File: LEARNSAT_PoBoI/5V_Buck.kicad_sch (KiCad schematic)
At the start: 22 parts, among them U8 LT1616ES6#TRMPBF, U9 LT1616ES6#TRMPBF

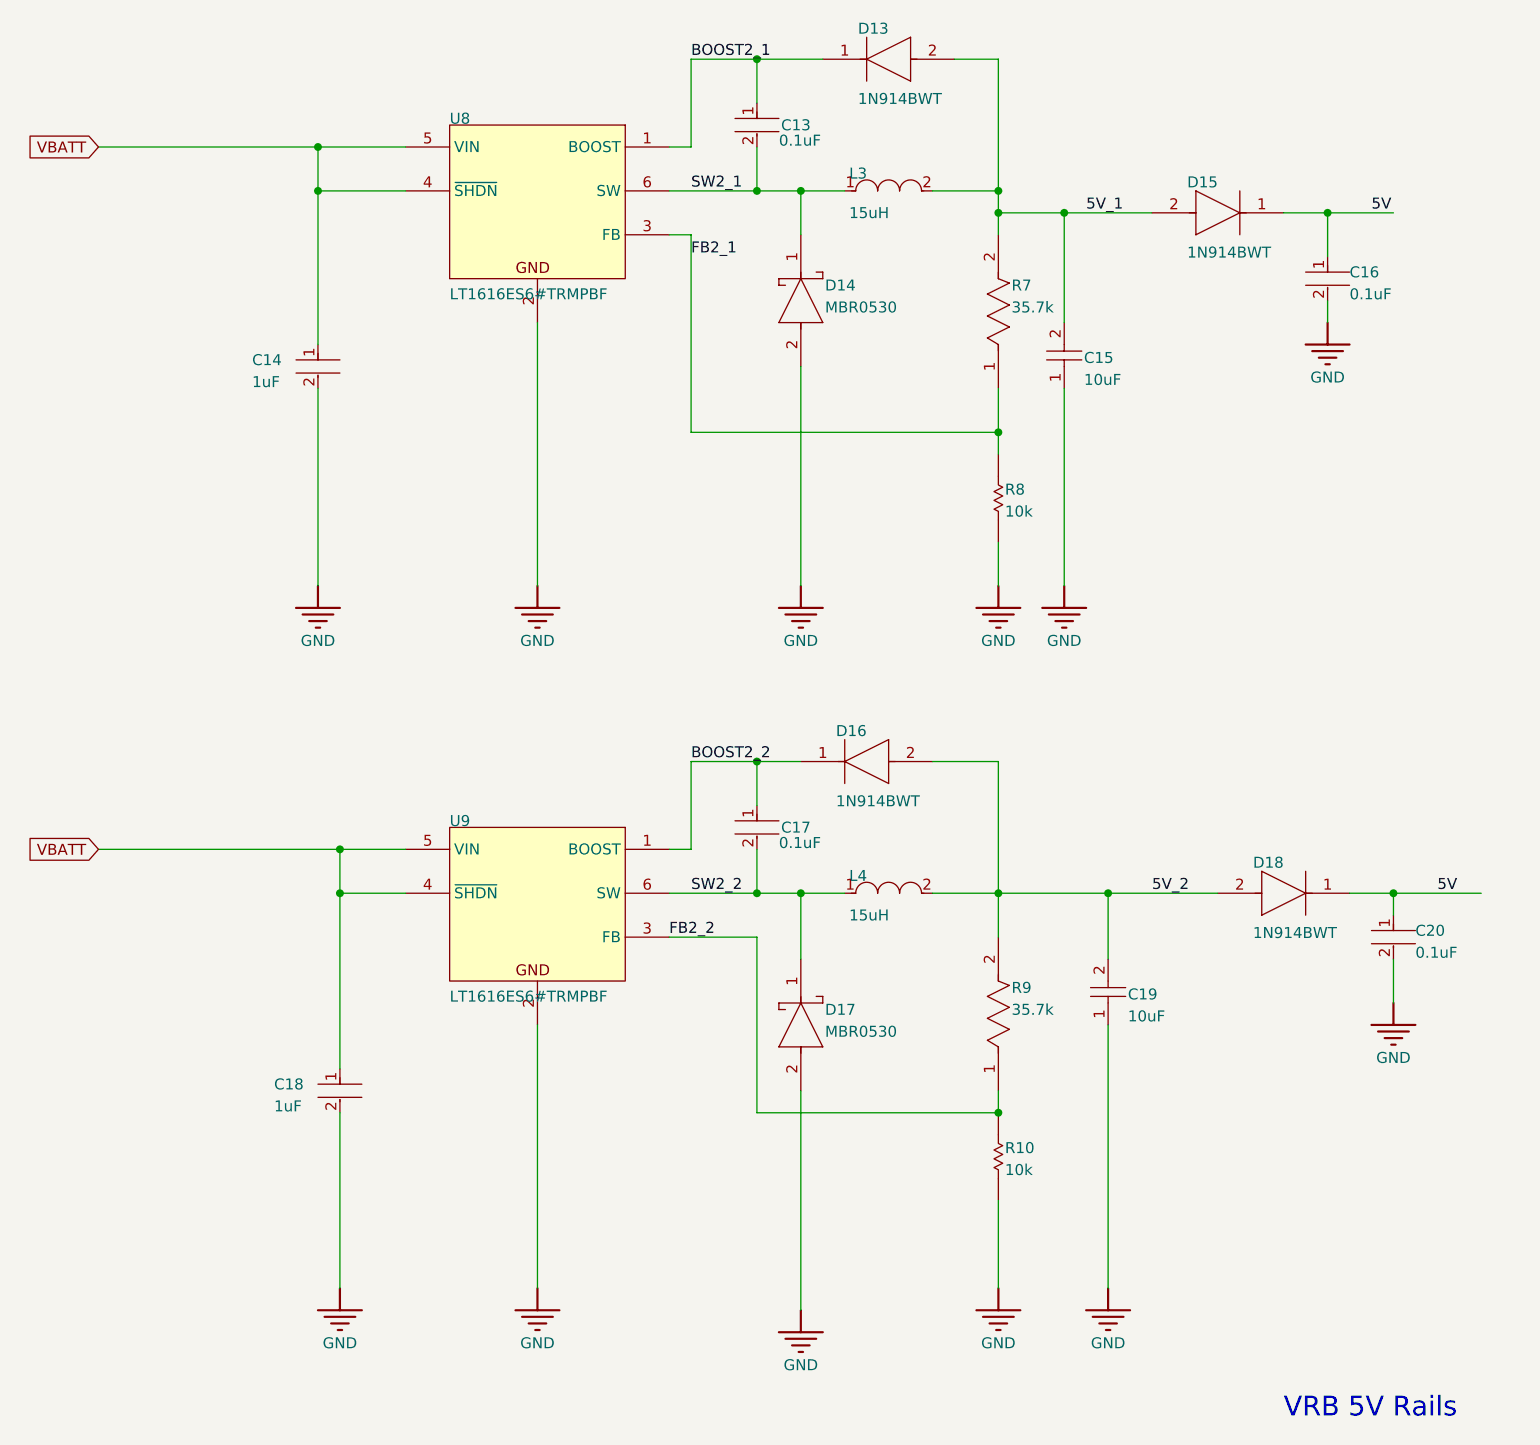
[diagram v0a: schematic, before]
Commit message: Added footprints
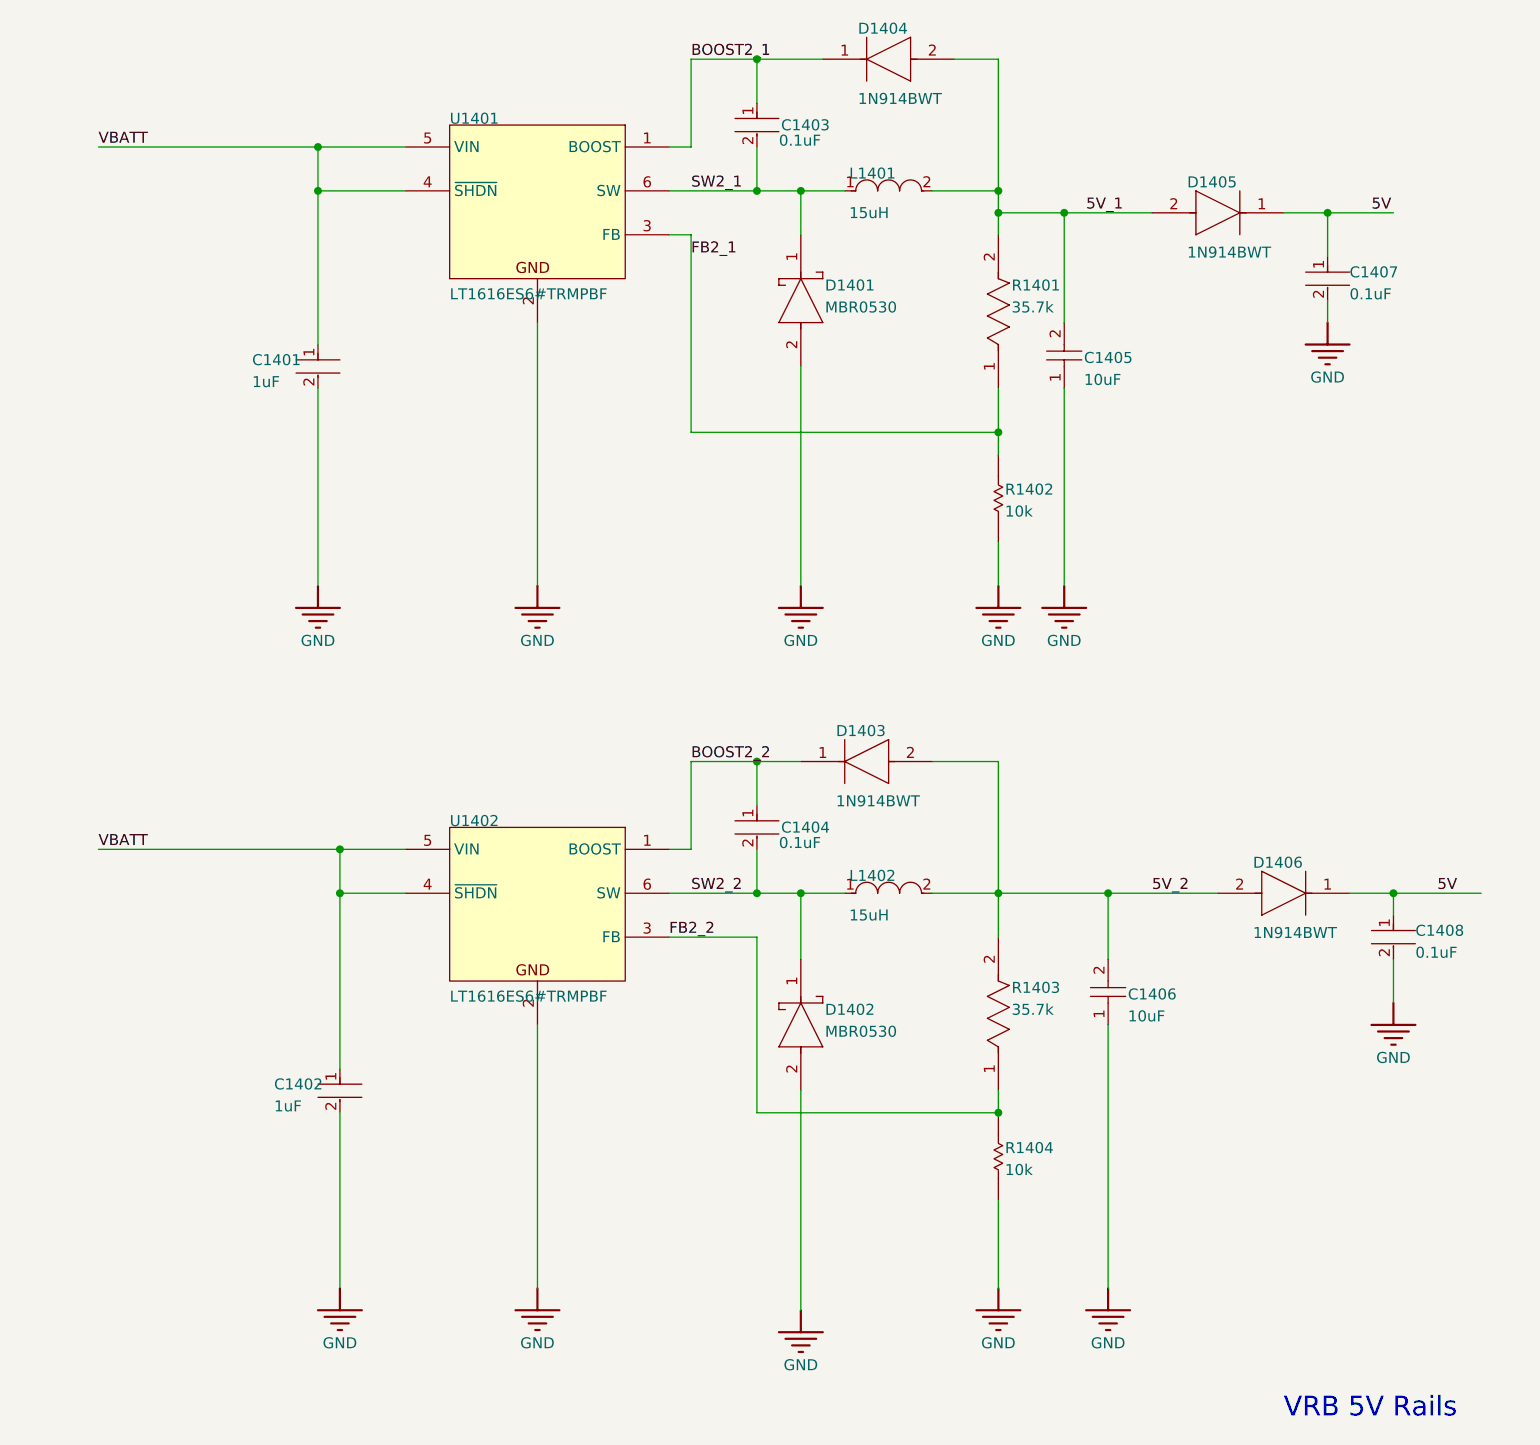
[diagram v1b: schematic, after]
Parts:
- C1401: renamed from C14; footprint FP-CL10-IPC_B -> Capacitor_SMD:C_0603_1608Metric
- C1402: renamed from C18; footprint FP-CL10-IPC_B -> Capacitor_SMD:C_0603_1608Metric
- C1403: renamed from C13; footprint FP-C0603-CJ-MFG -> Capacitor_SMD:C_0603_1608Metric
- C1404: renamed from C17; footprint FP-C0603-CJ-MFG -> Capacitor_SMD:C_0603_1608Metric
- C1405: renamed from C15; footprint CAPC0603(1608)100_L -> Capacitor_SMD:C_0603_1608Metric
- C1406: renamed from C19; footprint CAPC0603(1608)100_L -> Capacitor_SMD:C_0603_1608Metric
- C1407: renamed from C16; footprint FP-C0603-CJ-MFG -> Capacitor_SMD:C_0603_1608Metric
- C1408: renamed from C20; footprint FP-C0603-CJ-MFG -> Capacitor_SMD:C_0603_1608Metric
- D1401: renamed from D14; footprint FP-425-04-MFG -> Diode_SMD:D_SOD-123
- D1402: renamed from D17; footprint FP-425-04-MFG -> Diode_SMD:D_SOD-123
- D1403: renamed from D16; footprint FP-502-01-MFG -> Diode_SMD:D_SOD-123
- D1404: renamed from D13; footprint FP-502-01-MFG -> Diode_SMD:D_SOD-123
- D1405: renamed from D15; footprint FP-502-01-MFG -> Diode_SMD:D_SOD-123
- D1406: renamed from D18; footprint FP-502-01-MFG -> Diode_SMD:D_SOD-123
- L1401: renamed from L3; footprint FP-LQH43CN_03-MFG -> Inductor_SMD:L_1812_4532Metric
- L1402: renamed from L4; footprint FP-LQH43CN_03-MFG -> Inductor_SMD:L_1812_4532Metric
- R1401: renamed from R7; footprint FP-CRCW0603-e3-IPC_C -> Resistor_SMD:R_0603_1608Metric
- R1402: renamed from R8; footprint RESC1609X50X30NL8T20 -> Resistor_SMD:R_0603_1608Metric
- R1403: renamed from R9; footprint FP-CRCW0603-e3-IPC_C -> Resistor_SMD:R_0603_1608Metric
- R1404: renamed from R10; footprint RESC1609X50X30NL8T20 -> Resistor_SMD:R_0603_1608Metric
- U1401: renamed from U8; footprint LT-S6-6-SOT-23_M -> LT1616ES6TRMPBF:SOT-6_S
- U1402: renamed from U9; footprint LT-S6-6-SOT-23_M -> LT1616ES6TRMPBF:SOT-6_S

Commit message: Add files via upload
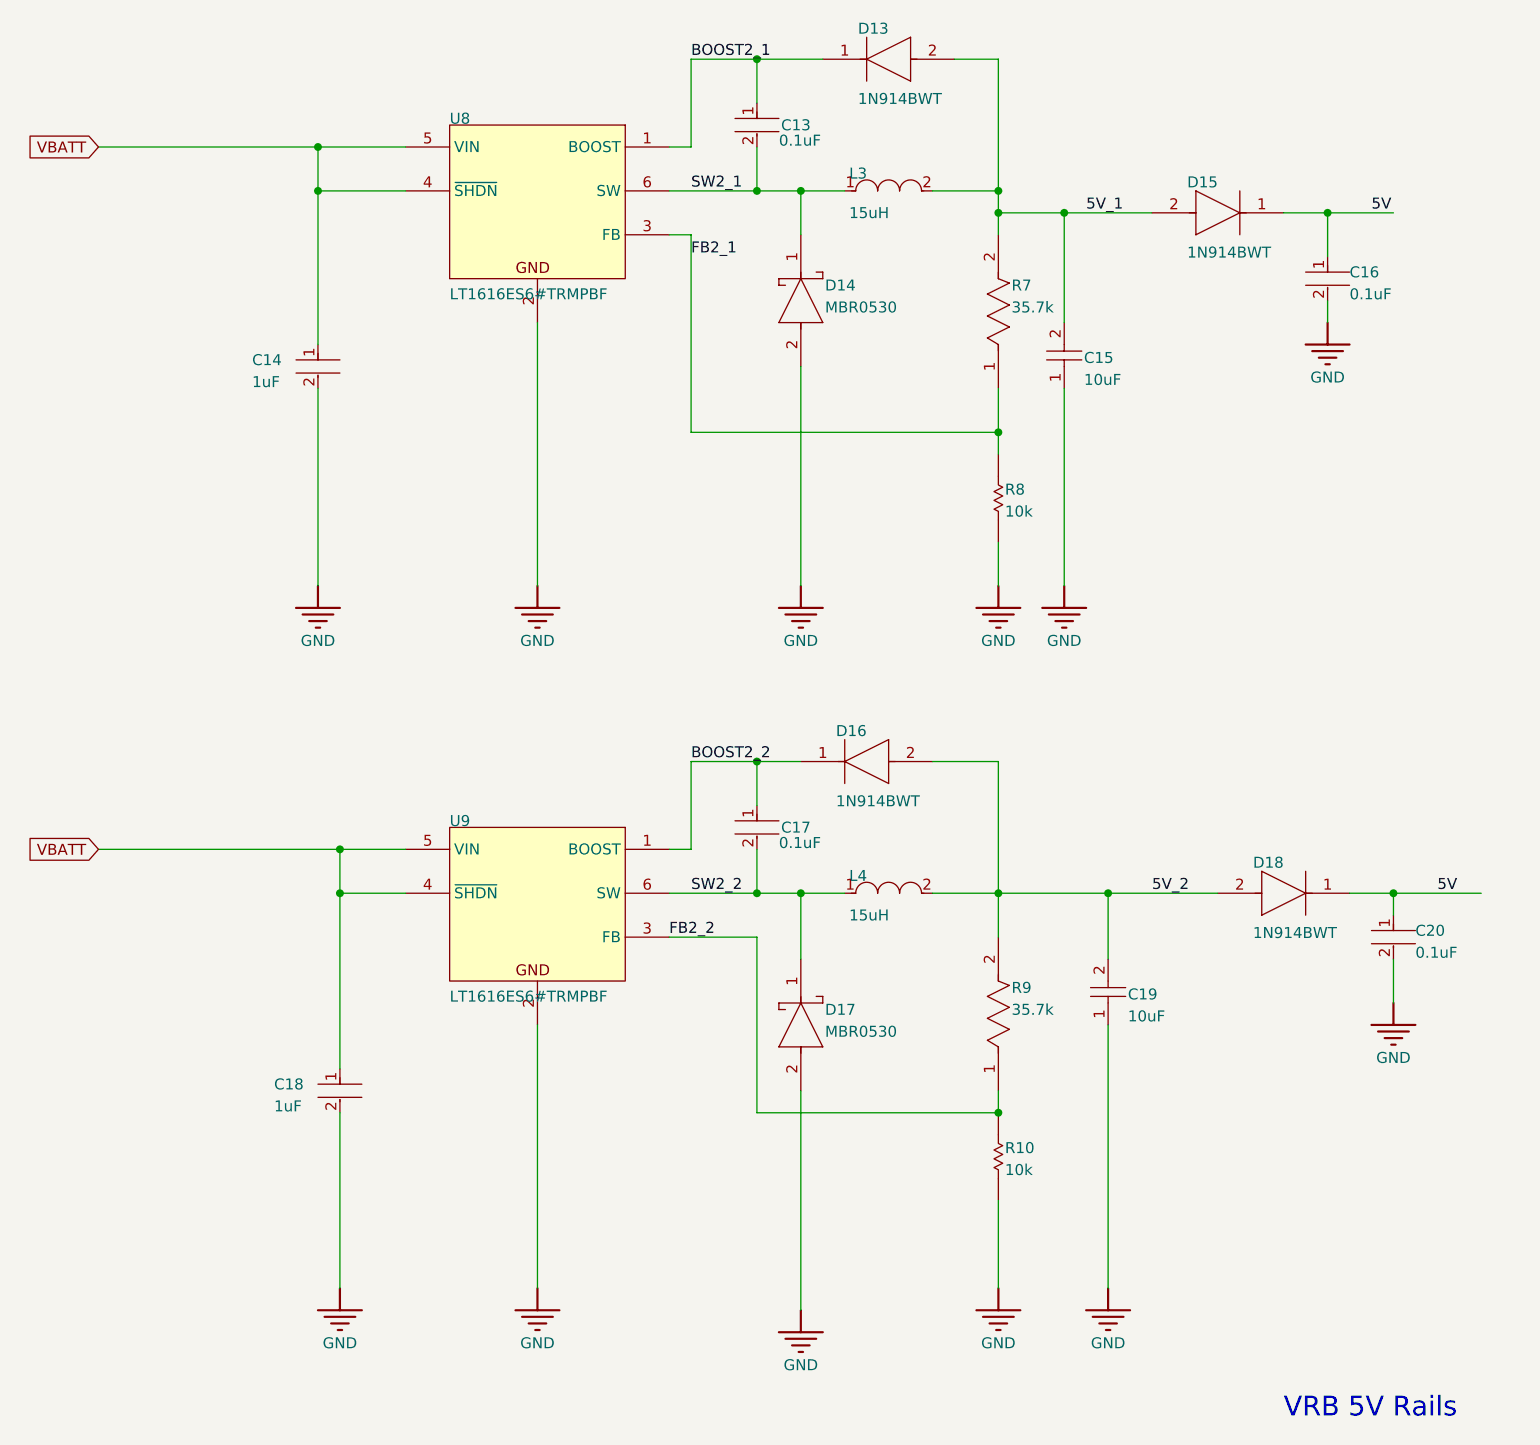
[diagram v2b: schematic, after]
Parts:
- C13: renamed from C1403; footprint Capacitor_SMD:C_0603_1608Metric -> FP-C0603-CJ-MFG
- C14: renamed from C1401; footprint Capacitor_SMD:C_0603_1608Metric -> FP-CL10-IPC_B
- C15: renamed from C1405; footprint Capacitor_SMD:C_0603_1608Metric -> CAPC0603(1608)100_L
- C16: renamed from C1407; footprint Capacitor_SMD:C_0603_1608Metric -> FP-C0603-CJ-MFG
- C17: renamed from C1404; footprint Capacitor_SMD:C_0603_1608Metric -> FP-C0603-CJ-MFG
- C18: renamed from C1402; footprint Capacitor_SMD:C_0603_1608Metric -> FP-CL10-IPC_B
- C19: renamed from C1406; footprint Capacitor_SMD:C_0603_1608Metric -> CAPC0603(1608)100_L
- C20: renamed from C1408; footprint Capacitor_SMD:C_0603_1608Metric -> FP-C0603-CJ-MFG
- D13: renamed from D1404; footprint Diode_SMD:D_SOD-123 -> FP-502-01-MFG
- D14: renamed from D1401; footprint Diode_SMD:D_SOD-123 -> FP-425-04-MFG
- D15: renamed from D1405; footprint Diode_SMD:D_SOD-123 -> FP-502-01-MFG
- D16: renamed from D1403; footprint Diode_SMD:D_SOD-123 -> FP-502-01-MFG
- D17: renamed from D1402; footprint Diode_SMD:D_SOD-123 -> FP-425-04-MFG
- D18: renamed from D1406; footprint Diode_SMD:D_SOD-123 -> FP-502-01-MFG
- L3: renamed from L1401; footprint Inductor_SMD:L_1812_4532Metric -> FP-LQH43CN_03-MFG
- L4: renamed from L1402; footprint Inductor_SMD:L_1812_4532Metric -> FP-LQH43CN_03-MFG
- R10: renamed from R1404; footprint Resistor_SMD:R_0603_1608Metric -> RESC1609X50X30NL8T20
- R7: renamed from R1401; footprint Resistor_SMD:R_0603_1608Metric -> FP-CRCW0603-e3-IPC_C
- R8: renamed from R1402; footprint Resistor_SMD:R_0603_1608Metric -> RESC1609X50X30NL8T20
- R9: renamed from R1403; footprint Resistor_SMD:R_0603_1608Metric -> FP-CRCW0603-e3-IPC_C
- U8: renamed from U1401; footprint LT1616ES6TRMPBF:SOT-6_S -> LT-S6-6-SOT-23_M
- U9: renamed from U1402; footprint LT1616ES6TRMPBF:SOT-6_S -> LT-S6-6-SOT-23_M
